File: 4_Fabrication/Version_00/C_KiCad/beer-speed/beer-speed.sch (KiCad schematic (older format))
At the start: 11 parts

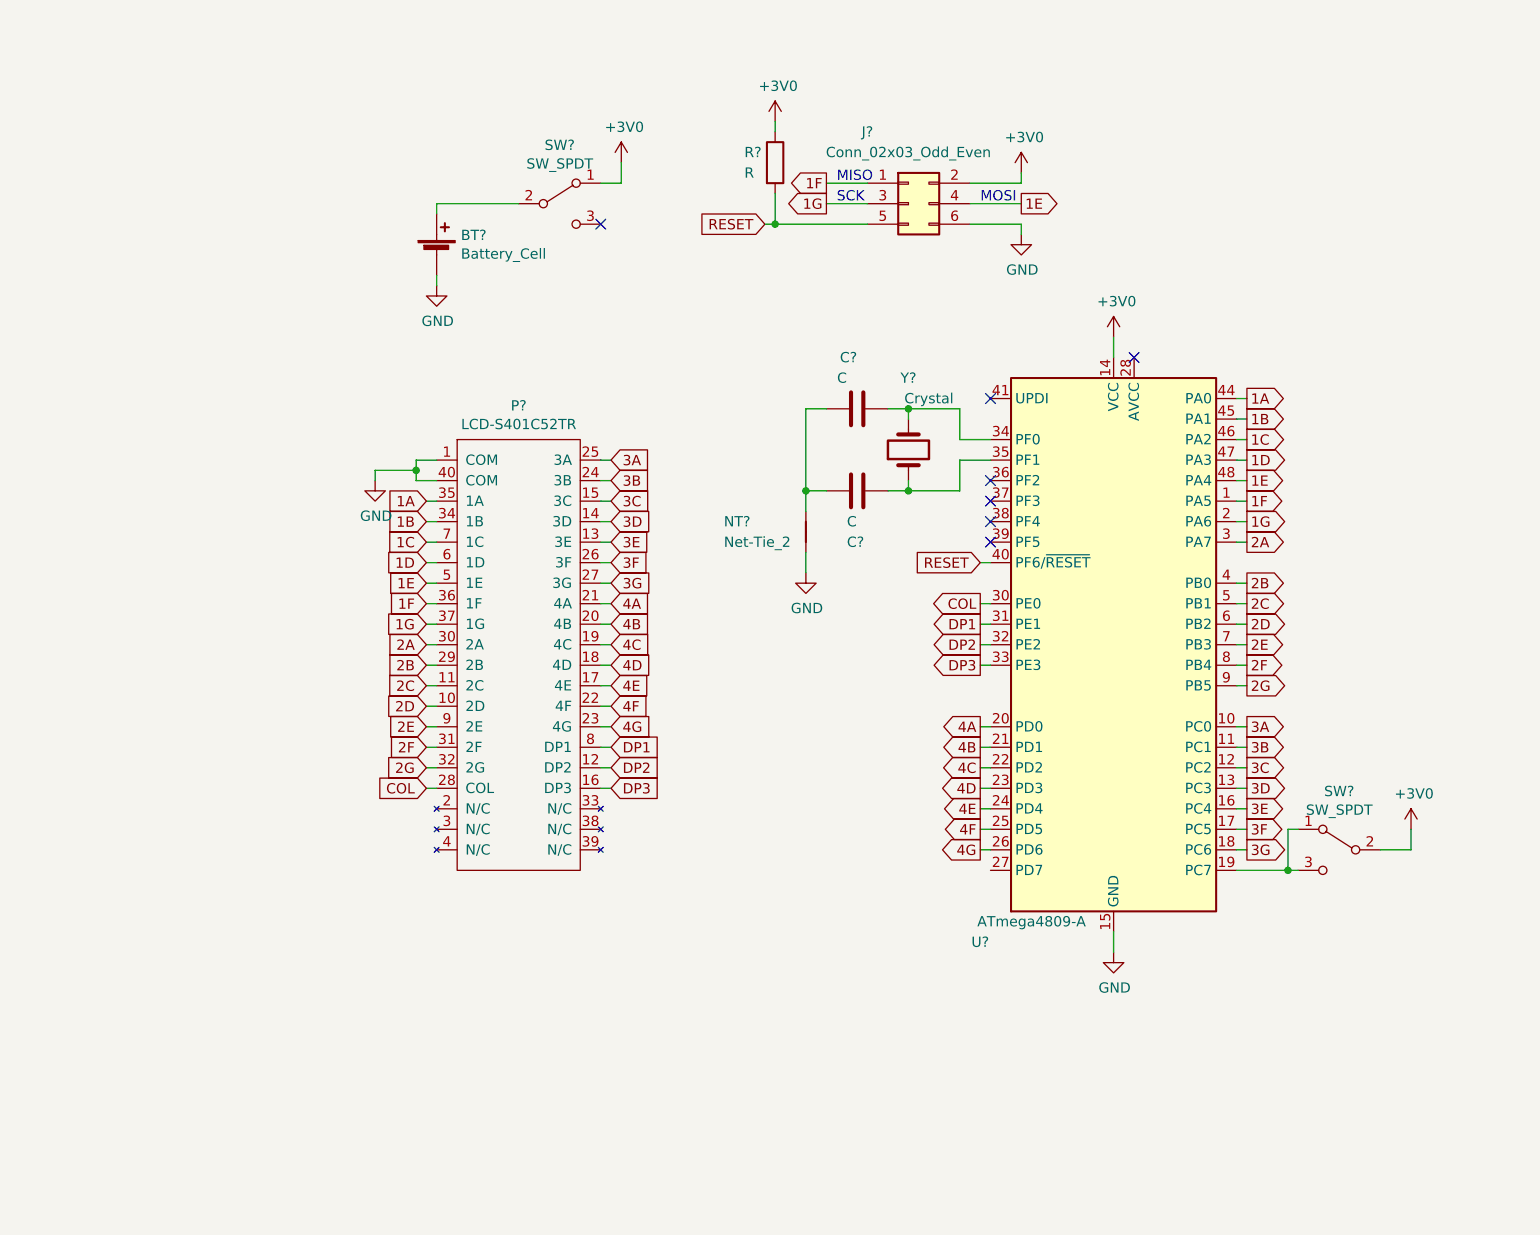
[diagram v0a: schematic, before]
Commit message: modif kicad
small modif
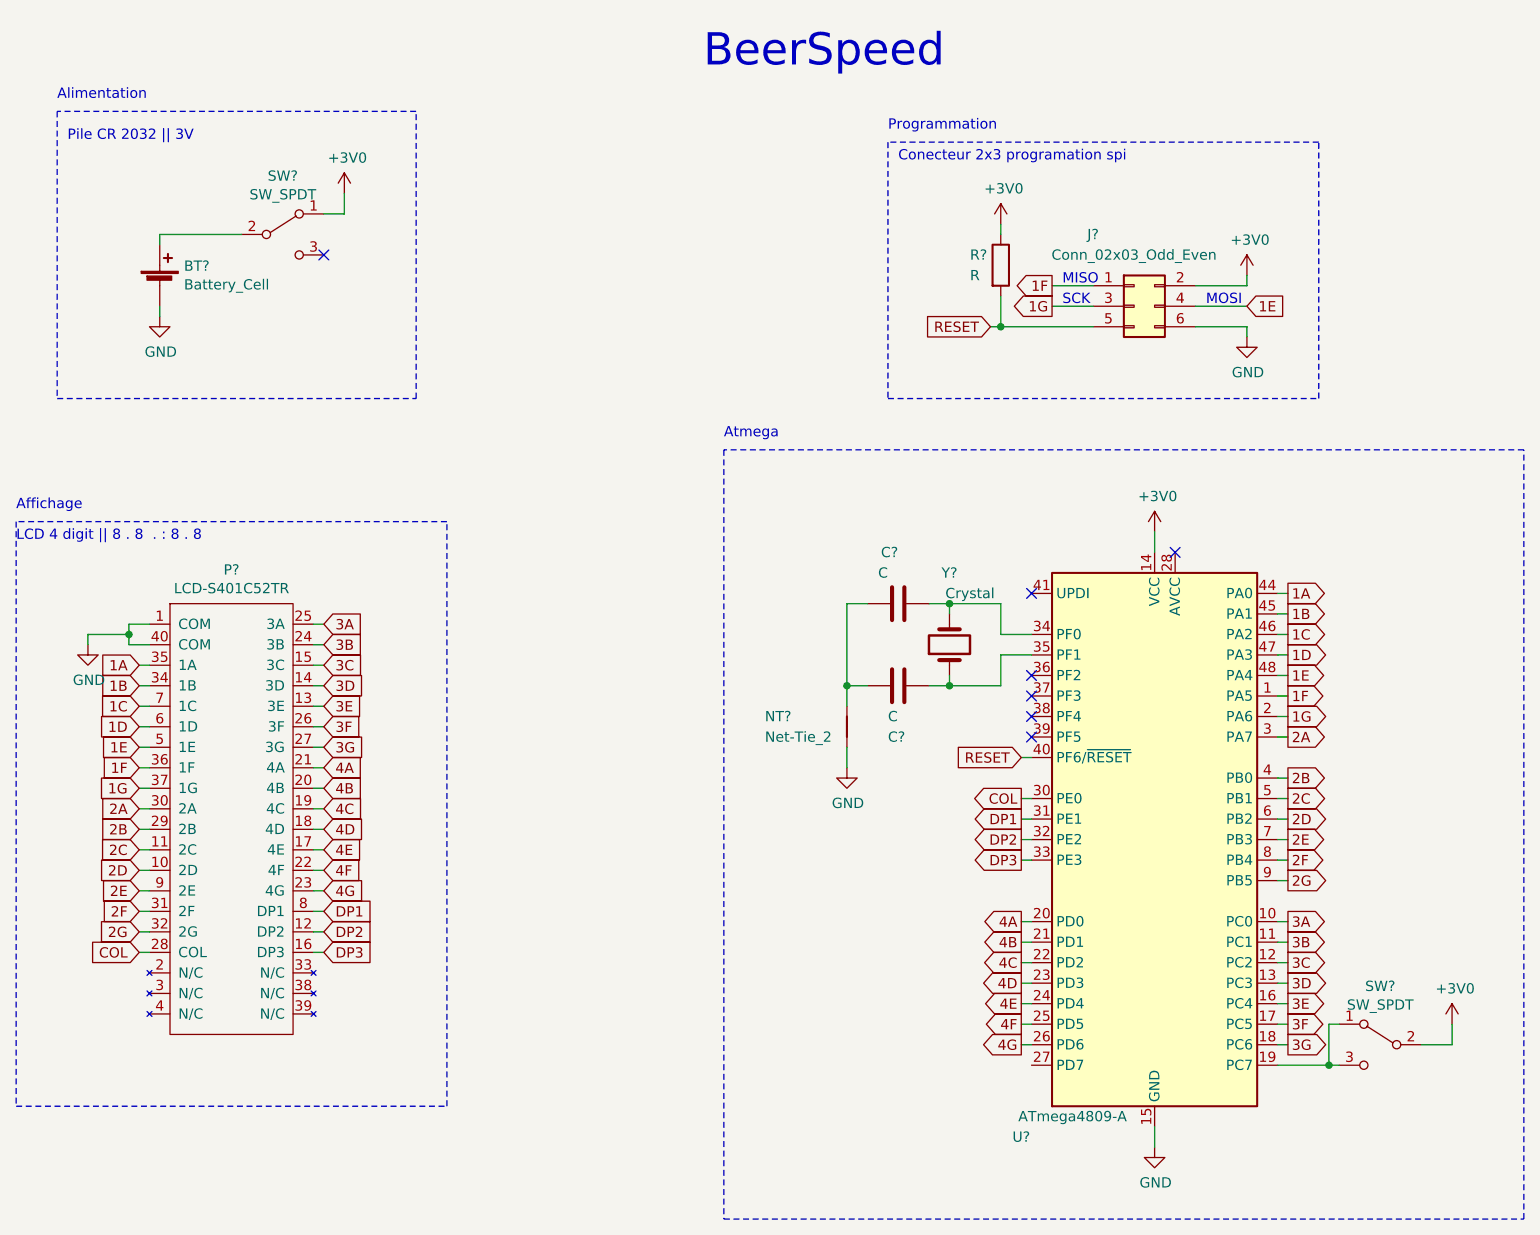
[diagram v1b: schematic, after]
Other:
- note added: "Affichage"
- note added: "Alimentation"
- note added: "Atmega\n"
- note added: "BeerSpeed"
- note added: "Conecteur 2x3 programation spi"
- note added: "LCD 4 digit || 8 . 8 . : 8 . 8"
- note added: "Pile CR 2032 || 3V"
- note added: "Programmation"
- moved on the sheet: BT?, C?, J?, NT?, P?, R?, SW?, U?, Y?
